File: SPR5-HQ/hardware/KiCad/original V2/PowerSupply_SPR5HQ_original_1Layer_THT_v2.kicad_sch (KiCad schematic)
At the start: 46 parts, among them J1 Screw_Terminal_01x02, J2 Screw_Terminal_01x02, J3 Screw_Terminal_01x02, J4 Screw_Terminal_01x02, U1 LM338, U2 LM338

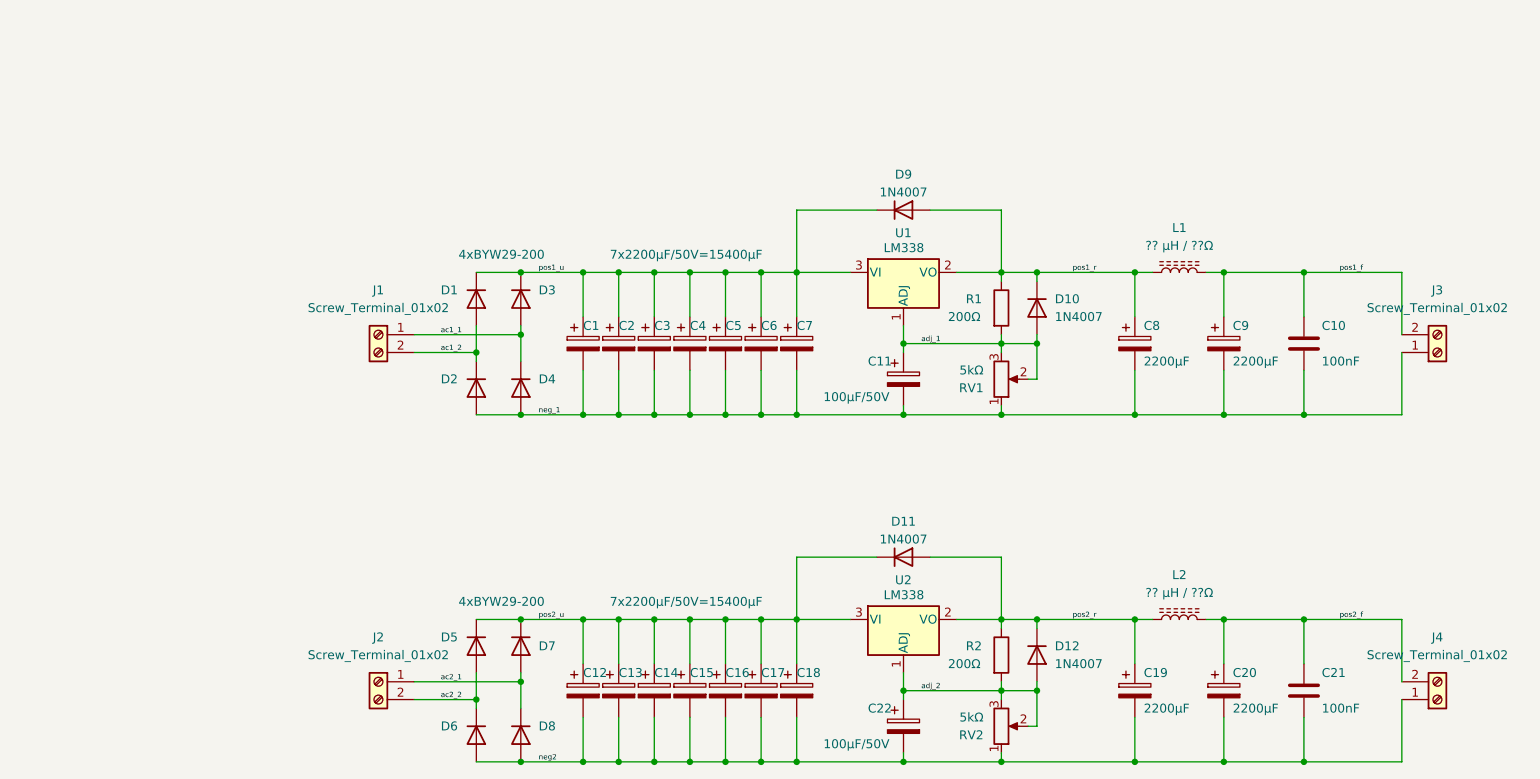
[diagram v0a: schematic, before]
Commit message: Add files via upload
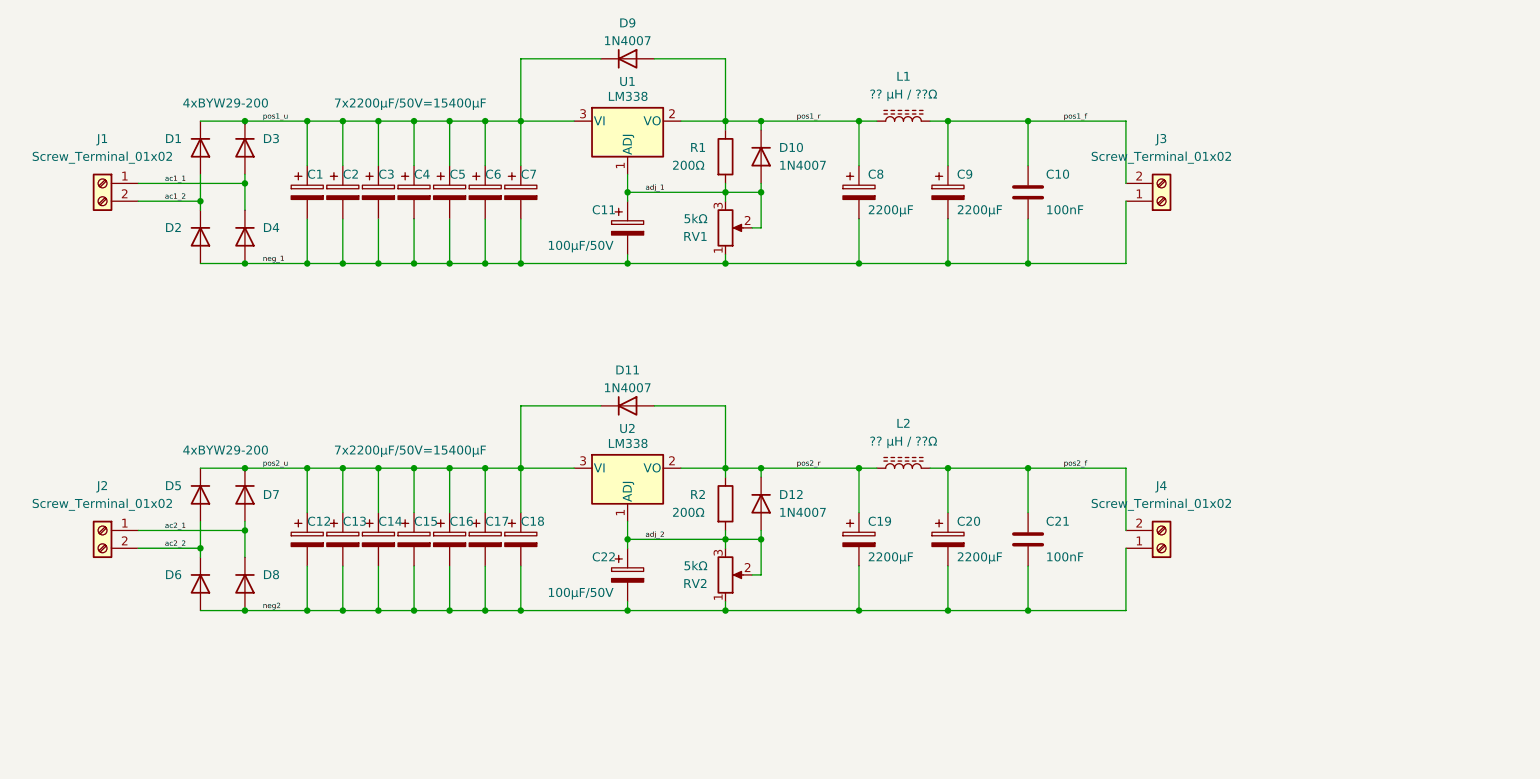
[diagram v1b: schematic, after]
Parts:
- D10, D12: footprint analoghifi:D_DO-41_SOD81_P10.16mm_Horizontal_minSilk -> analoghifi:D_DO-41_SOD81_short_P9.0mm_Horiz_minSilk
- R1, R2: footprint analoghifi:R_Axial_DIN0207_L6.3mm_D2.5mm_P10.16mm_Horizontal_minSilk -> analoghifi:R_Axial_Short_L6.3mm_D2.5mm_P9.0mm_Horiz_minSilk
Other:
- moved on the sheet: C1, C10, C11, C12, C13, C14, C15, C16, C17, C18, C19, C2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
